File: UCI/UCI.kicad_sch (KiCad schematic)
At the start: 8 parts, among them J1 USB_C_Receptacle, U1 ESD224DQA

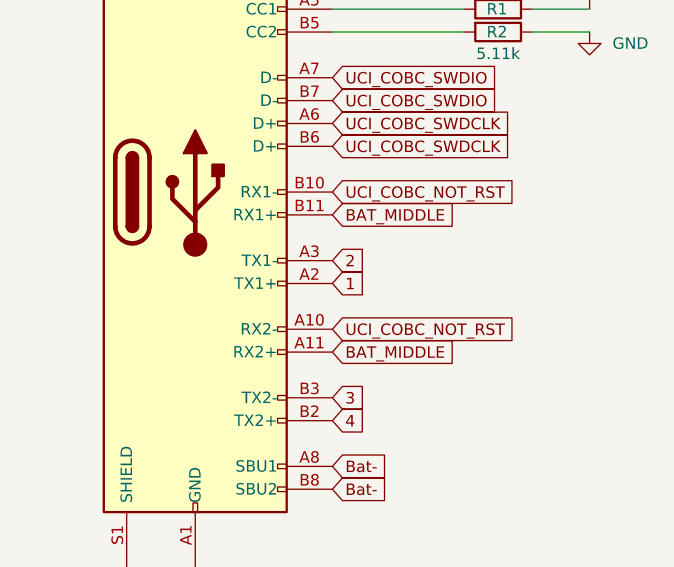
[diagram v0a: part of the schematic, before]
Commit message: Commit before the order.
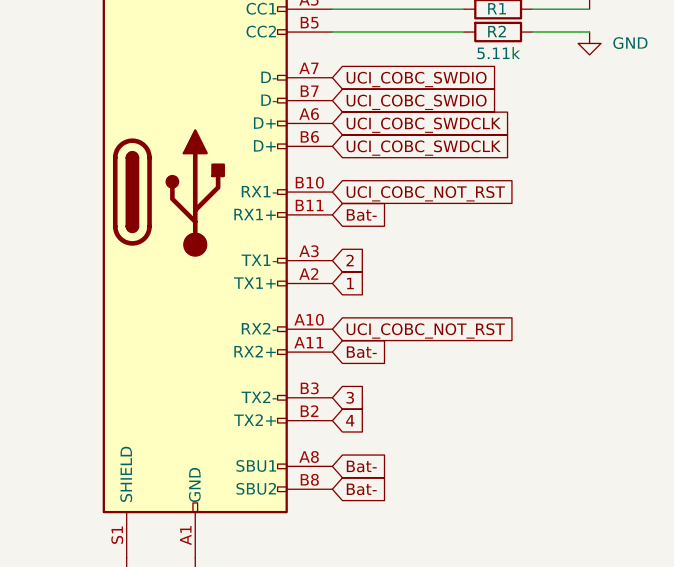
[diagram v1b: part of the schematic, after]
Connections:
- net BAT_MIDDLE is gone; now on net Bat-: J1.A11 (RX2+), J1.B11 (RX1+)
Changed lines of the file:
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@@
-    )
-  )
-  (global_label "BAT_MIDDLE" (shape input) (at 143.51 97.155 0) (fields_autoplaced)
-    (effects (font (size 1.27 1.27)) (justify left))
-    (property "Intersheetrefs" "${INTERSHEET_REFS}" (at 157.5623 97.155 0)
-      (effects (font (size 1.27 1.27)) (justify left) hide)
     )
   )
@@
     )
   )
-  (global_label "BAT_MIDDLE" (shape input) (at 143.51 112.395 0) (fields_autoplaced)
+  (global_label "Bat-" (shape input) (at 143.51 97.155 0) (fields_autoplaced)
     (effects (font (size 1.27 1.27)) (justify left))
-    (property "Intersheetrefs" "${INTERSHEET_REFS}" (at 157.5623 112.395 0)
+    (property "Intersheetrefs" "${INTERSHEET_REFS}" (at 151.2123 97.155 0)
       (effects (font (size 1.27 1.27)) (justify left) hide)
     )
@@
       (effects (font (size 1.27 1.27)) (justify left) hide)
     )
+  )
+  (global_label "Bat-" (shape input) (at 143.51 112.395 0) (fields_autoplaced)
+    (effects (font (size 1.27 1.27)) (justify left))
+    (property "Intersheetrefs" "${INTERSHEET_REFS}" (at 151.2123 112.395 0)
+      (effects (font (size 1.27 1.27)) (justify left) hide)
+    )
